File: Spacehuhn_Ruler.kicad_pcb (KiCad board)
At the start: 2 copper layers, 150 x 25 mm, 47 parts

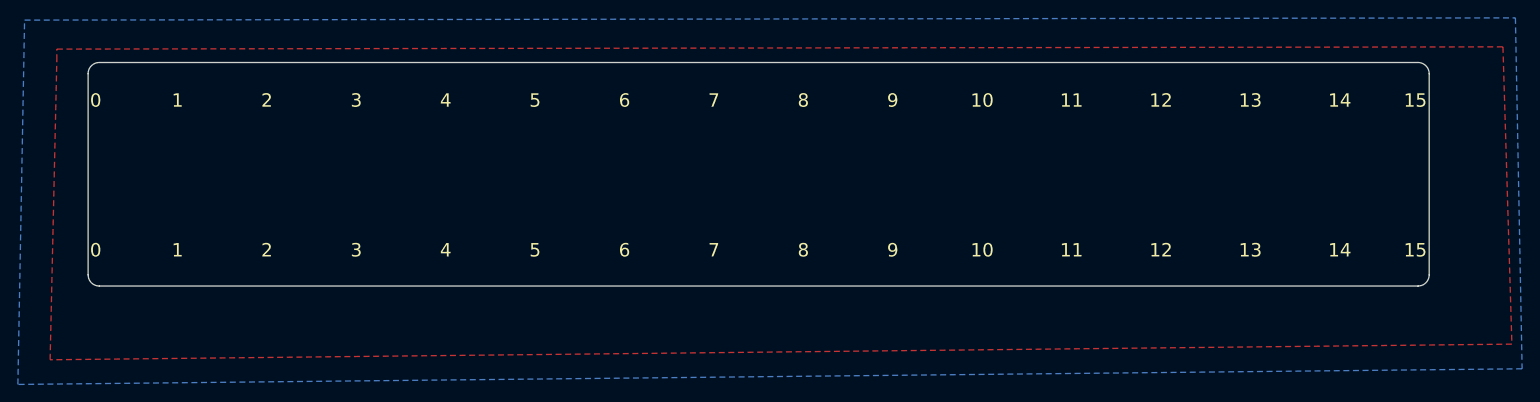
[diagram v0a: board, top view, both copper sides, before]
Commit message: Made it exactly 1 inch in height
For the memes (sorry americans)
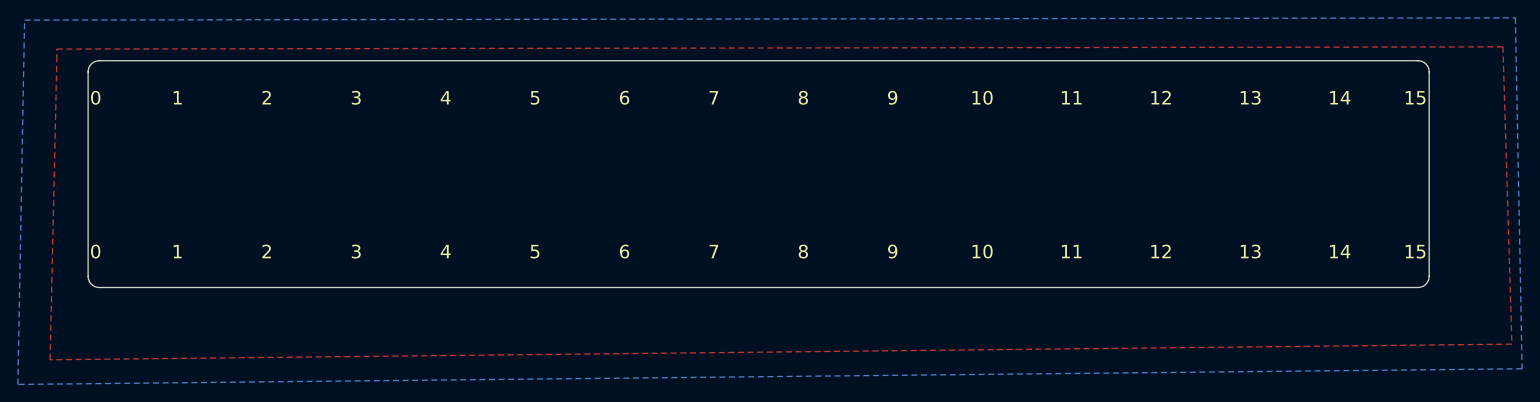
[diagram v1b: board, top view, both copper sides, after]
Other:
- board size 150 x 25 mm -> 150 x 25.4 mm
- board text added: "it 1 inch lol"
